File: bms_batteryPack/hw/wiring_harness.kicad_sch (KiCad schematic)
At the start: 5 parts, among them J1 Conn_01x02_Pin, SW1 SW_Push

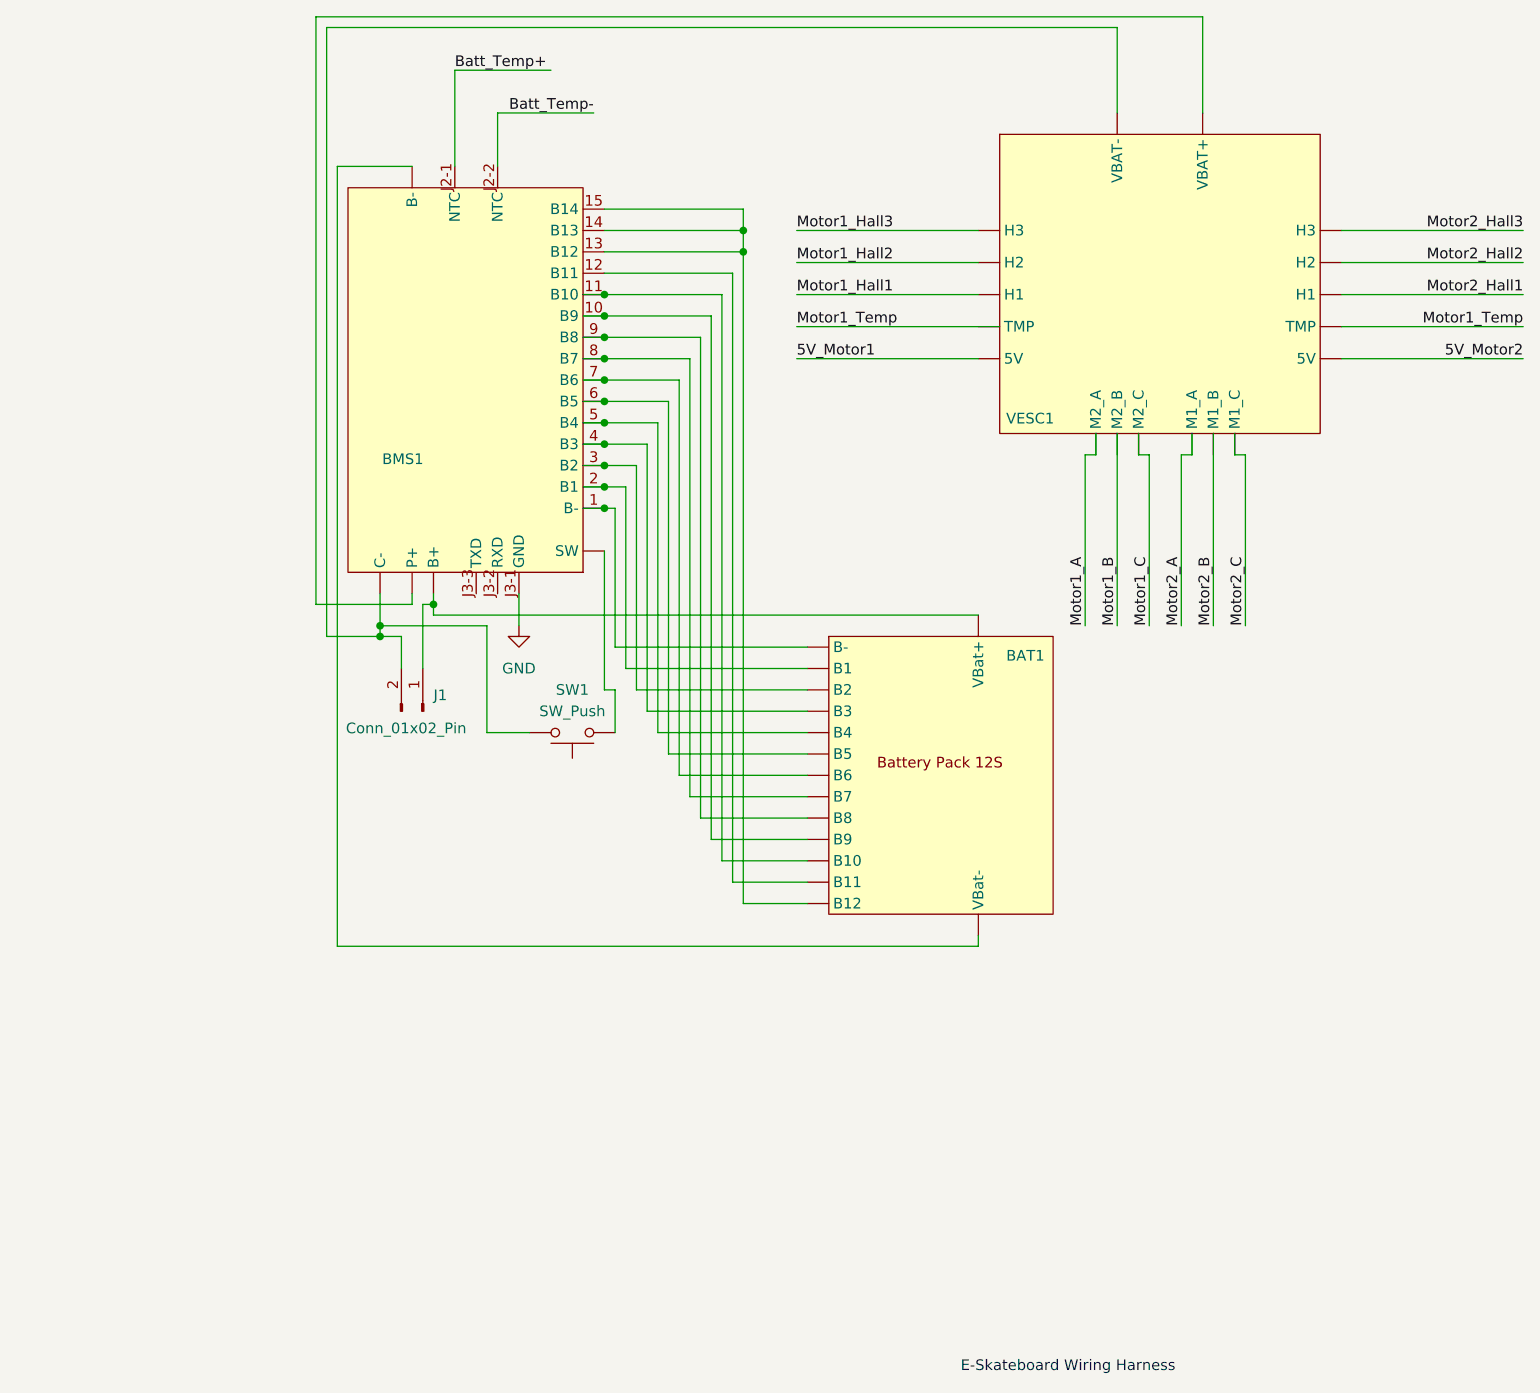
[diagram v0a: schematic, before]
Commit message: Updated with VESC receiver and button
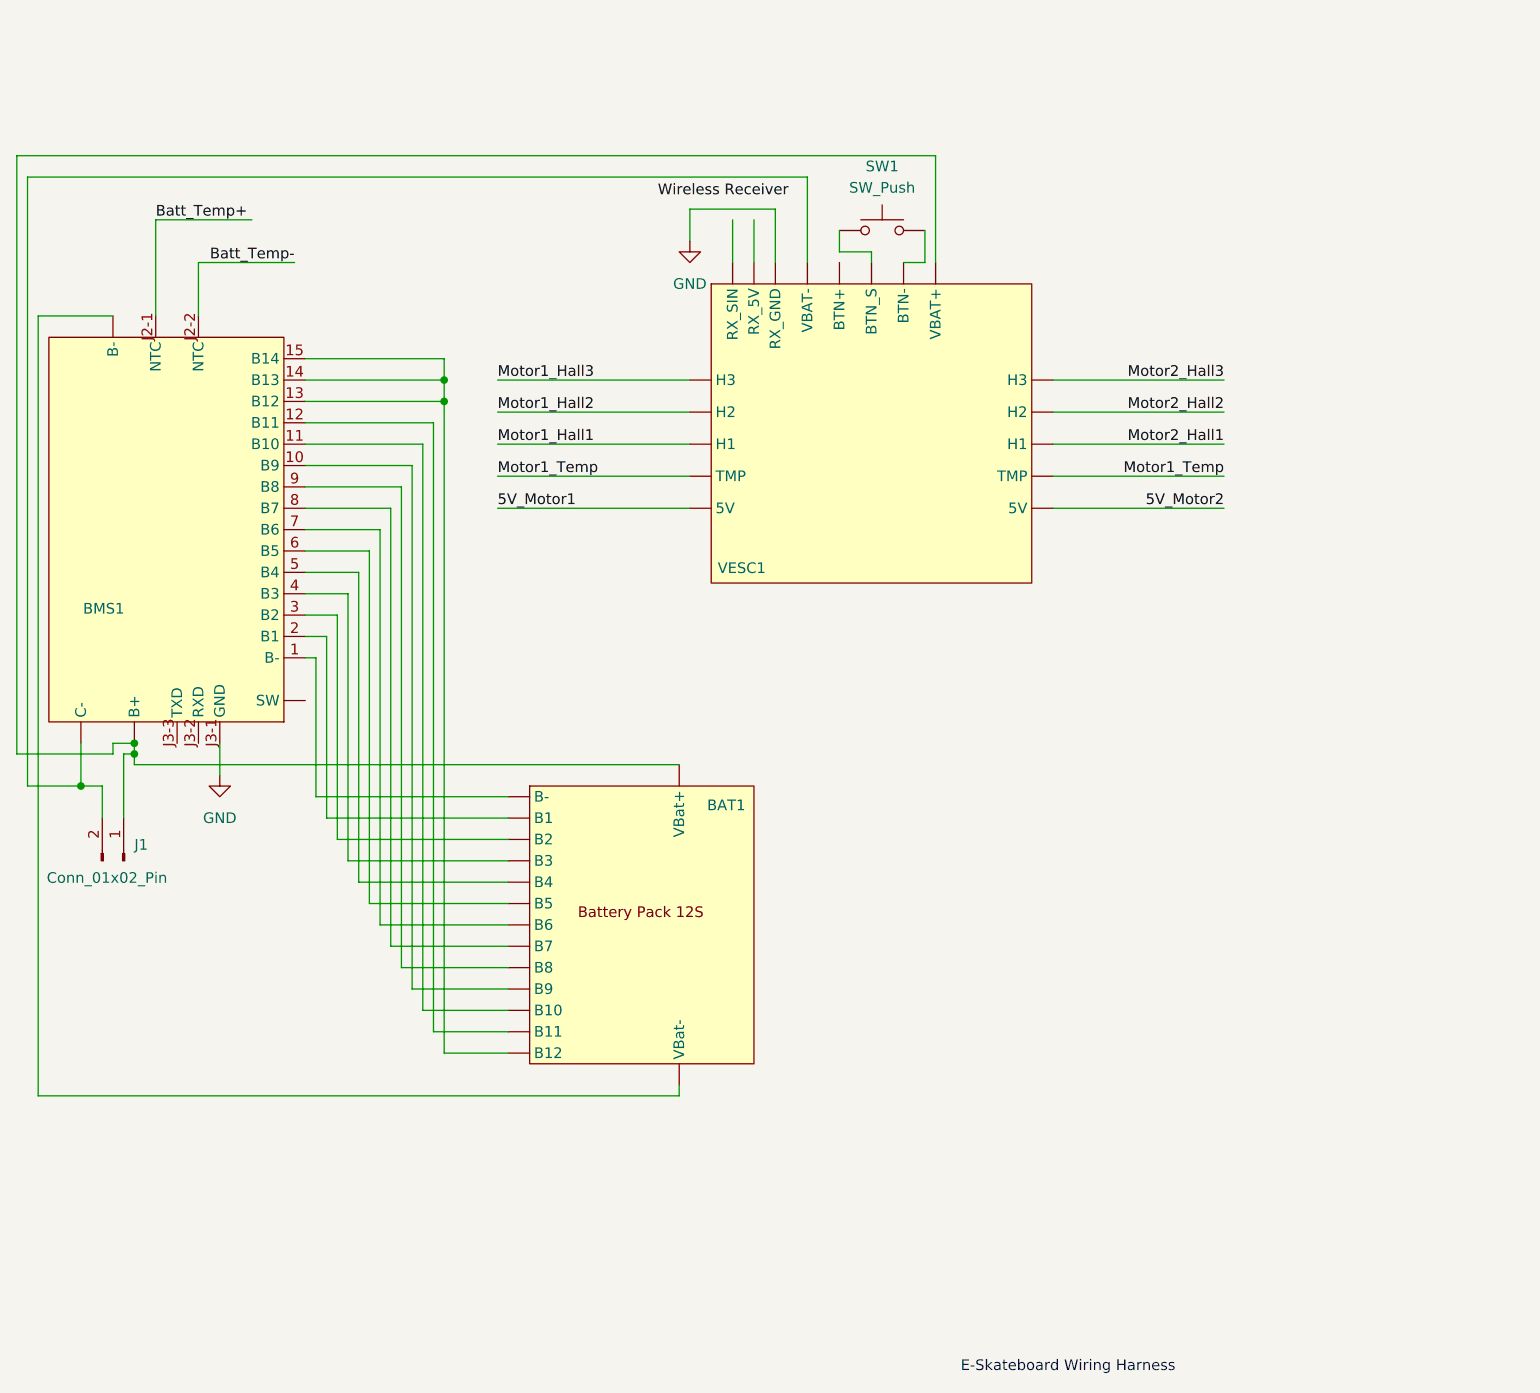
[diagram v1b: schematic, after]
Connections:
- net Motor1_A is gone; now on net Motor2_Hall3: VESC1. (5V)
- net Motor1_C is gone; now on net Motor2_Hall3: VESC1. (5V)
- net Motor2_A is gone; now on net Motor2_Hall3: VESC1. (5V)
- net Motor2_C is gone; now on net Motor2_Hall3: VESC1. (5V)
- net GND: now also VESC1. (5V)
- net at BAT1. (VBat-): now also BMS1.9 (B8); no longer BMS1. (C-)
- net at BMS1. (C-), J1.2 (Pin_2), VESC1. (5V): no longer SW1.2
- net at SW1.1: now also VESC1. (5V); no longer BMS1. (C-)
- new net: BAT1. (VBat-), BMS1. (C-)
- new net: BAT1. (VBat-), BMS1. (C-), J1.1 (Pin_1), VESC1. (5V)
- new net: SW1.2, VESC1. (5V)
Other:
- moved on the sheet: BAT1, J1, SW1, VESC1
